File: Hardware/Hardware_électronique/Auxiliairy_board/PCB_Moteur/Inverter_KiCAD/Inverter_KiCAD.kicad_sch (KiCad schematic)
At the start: 67 parts, among them J1 Conn_02x02_Top_Bottom, J2 173010542, J3 Conn_02x05_Odd_Even, J4 Conn_01x02, J5 Conn_01x02, Q5 SQ2310ES, U1 MIC4606, U2 GO 10-SME/SP3, U3 GO 10-SME/SP3, U4 AZ1117-3.3, U5 MAX3097ECSE+, U7 CSD86350Q5D, U8 CSD86350Q5D

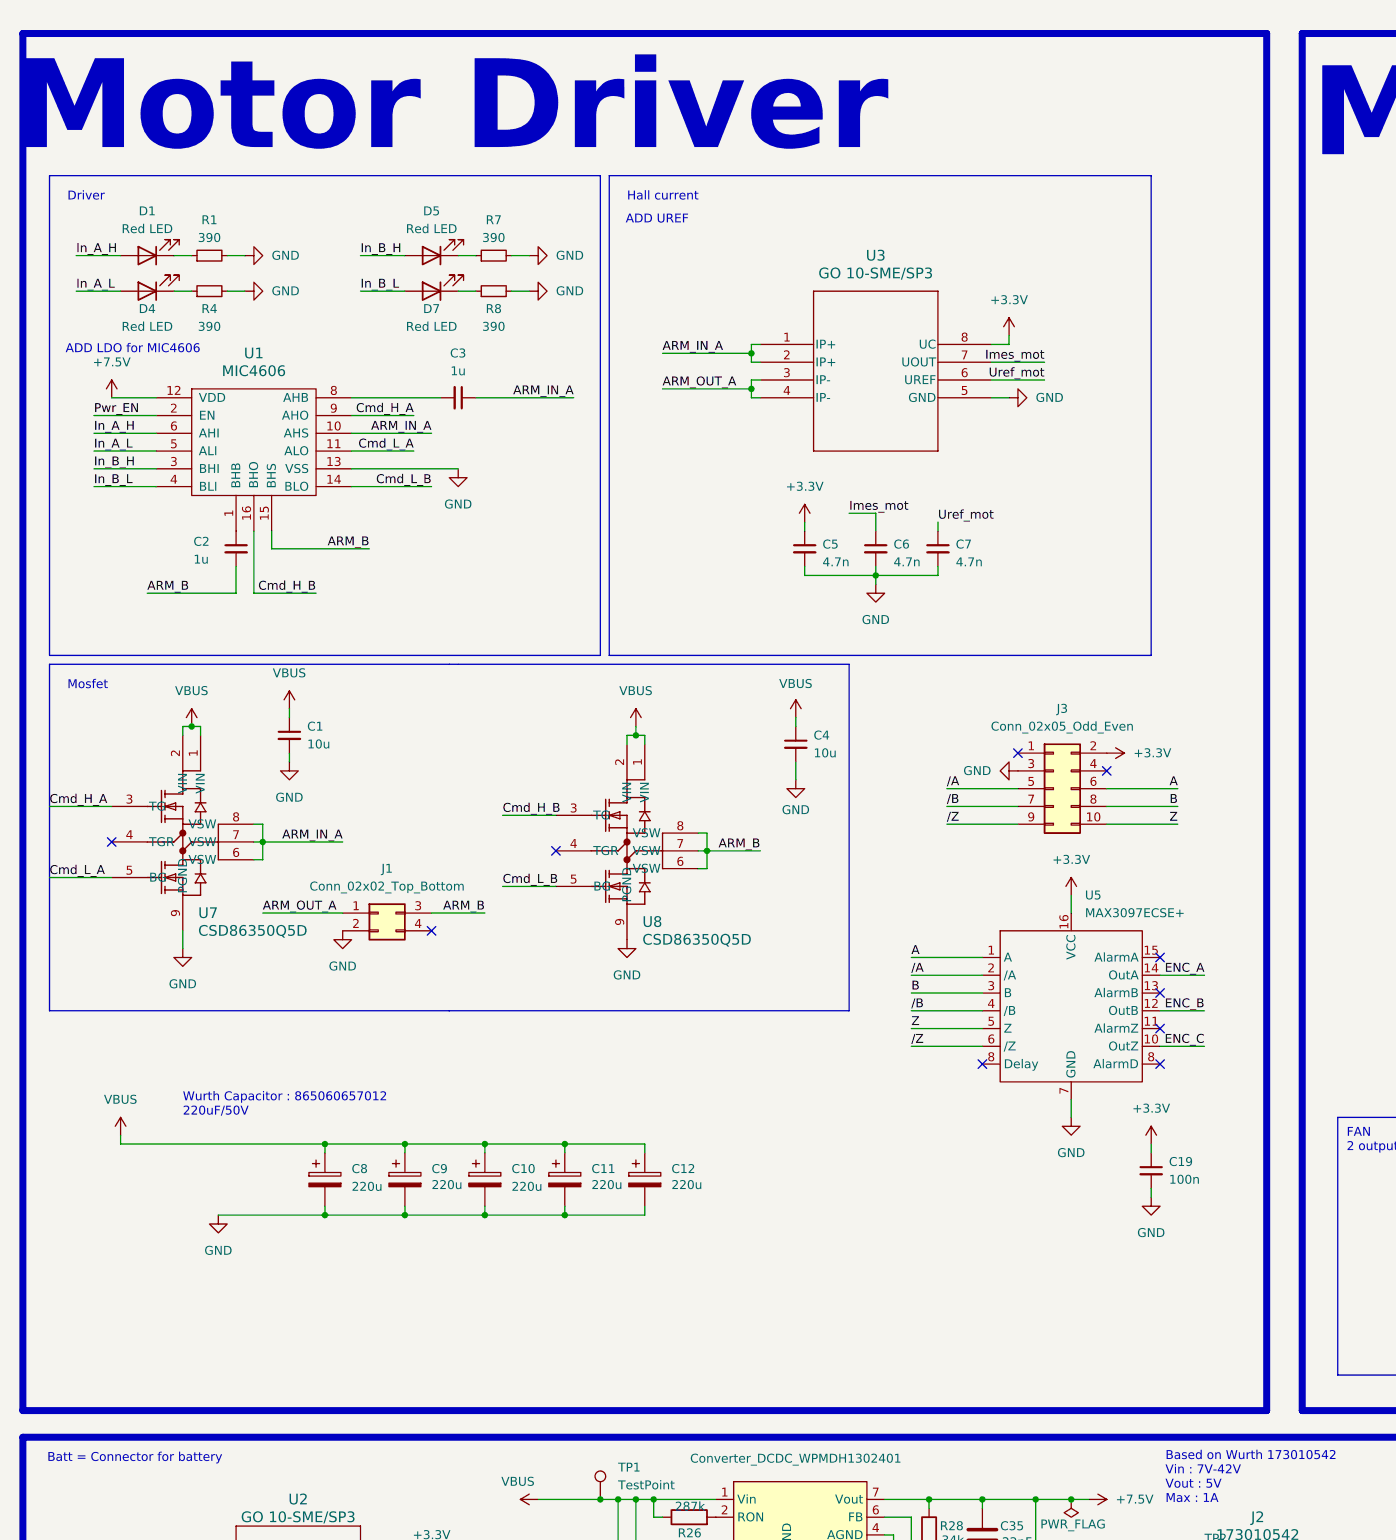
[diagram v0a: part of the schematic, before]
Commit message: ey
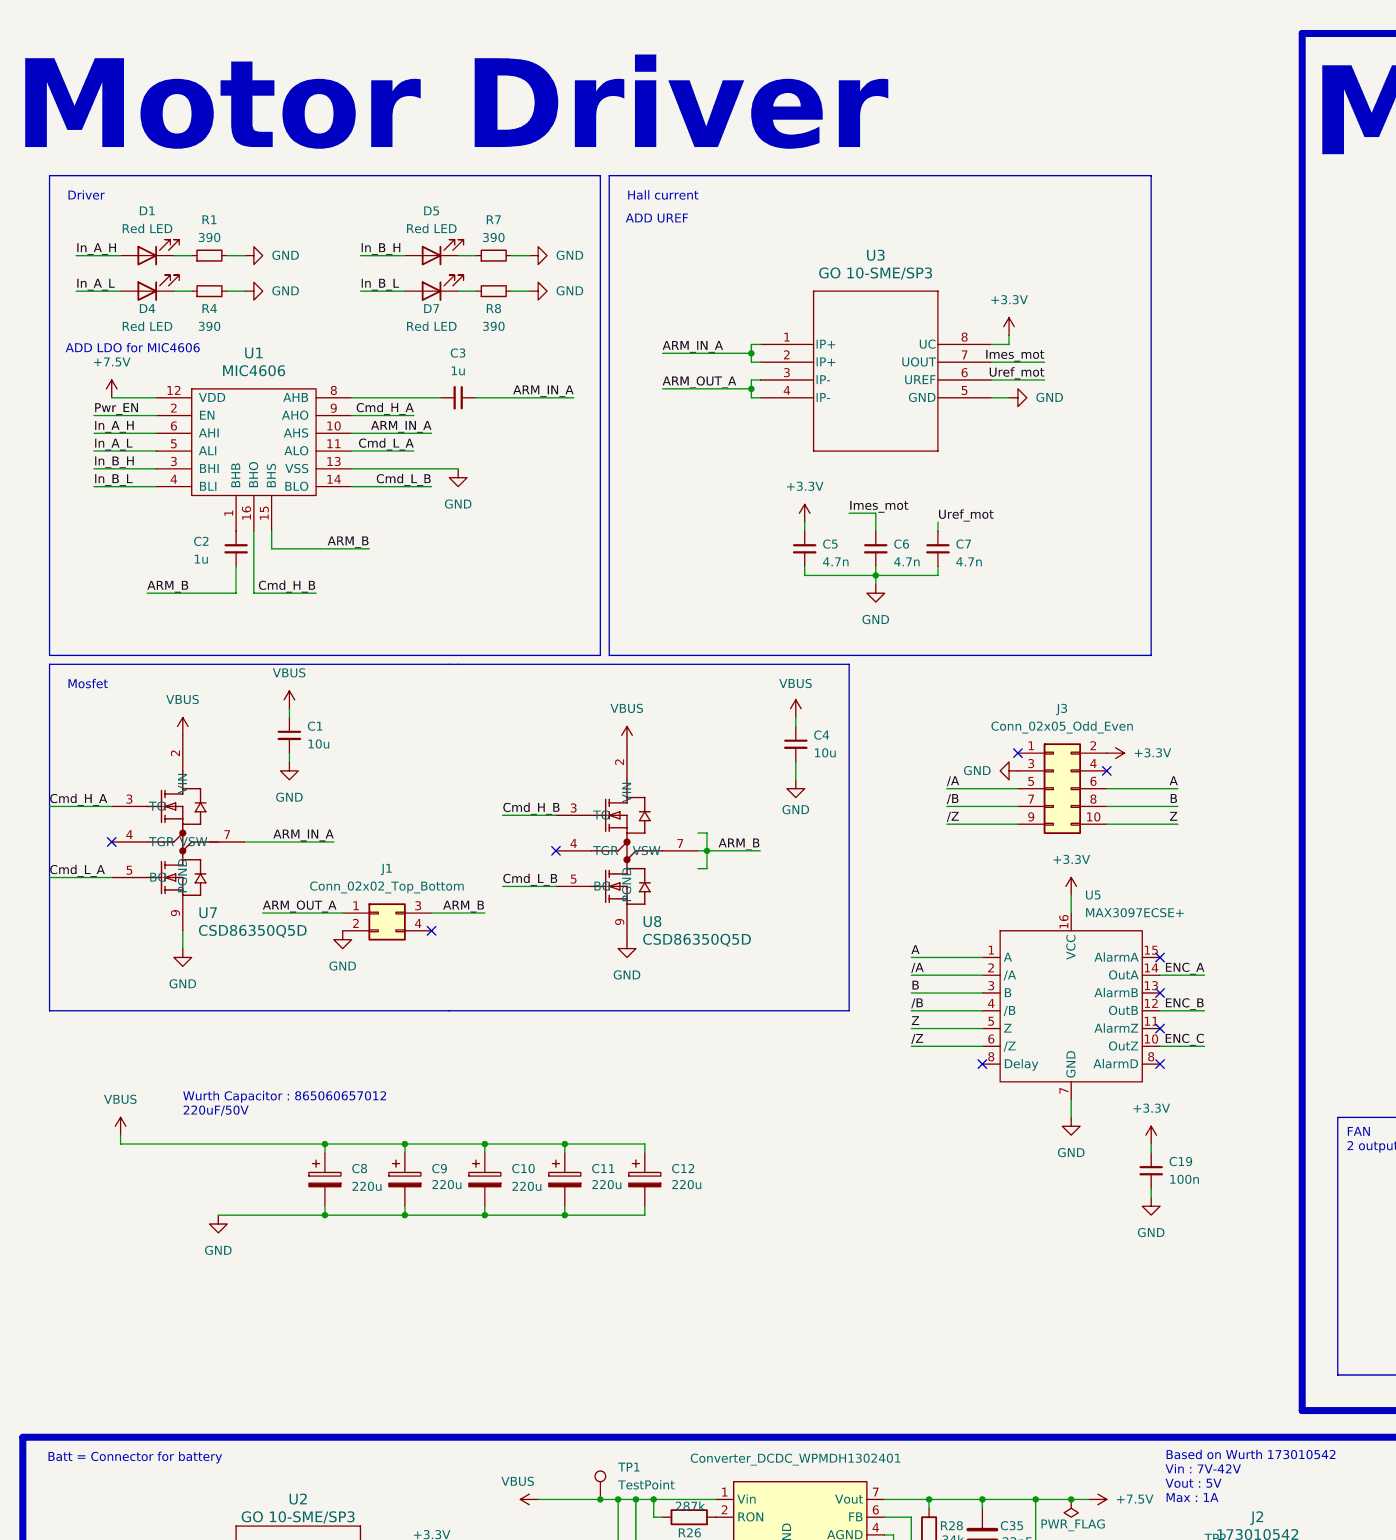
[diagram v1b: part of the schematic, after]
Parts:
- BT1: footprint Connector_AMASS:AMASS_XT60-F_1x02_P7.20mm_Vertical -> Connector_AMASS:AMASS_XT60-M_1x02_P7.20mm_Vertical
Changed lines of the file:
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@@
 	)
 	(junction
-		(at 102.87 114.3)
-		(diameter 0)
-		(color 0 0 0 0)
-	)
-	(junction
 		(at 92.71 172.72)
 		(diameter 0)
@@
 	)
 	(junction
-		(at 49.53 129.54)
-		(diameter 0)
-		(color 0 0 0 0)
-	)
-	(junction
 		(at 58.42 172.72)
 		(diameter 0)
@@
 	)
 	(junction
-		(at 39.37 113.03)
-		(diameter 0)
-		(color 0 0 0 0)
-	)
-	(junction
 		(at 332.74 241.3)
 		(diameter 0)
@@
 	(wire
 		(pts
-			(xy 40.64 113.03) (xy 40.64 114.3)
-		)
-		(stroke
-			(width 0)
-			(type default)
-		)
-	)
-	(wire
-		(pts
-			(xy 48.26 129.54) (xy 49.53 129.54)
+			(xy 46.99 129.54) (xy 59.69 129.54)
 		)
 		(stroke
@@
 	(wire
 		(pts
-			(xy 38.1 114.3) (xy 38.1 113.03)
-		)
-		(stroke
-			(width 0)
-			(type default)
-		)
-	)
-	(wire
-		(pts
 			(xy 252.73 181.61) (xy 254 181.61)
 		)
@@
 	(wire
 		(pts
-			(xy 49.53 129.54) (xy 60.96 129.54)
-		)
-		(stroke
-			(width 0)
-			(type default)
-		)
-	)
-	(wire
-		(pts
 			(xy 320.04 222.25) (xy 320.04 226.06)
 		)
@@
 	(wire
 		(pts
-			(xy 104.14 114.3) (xy 104.14 115.57)
-		)
-		(stroke
-			(width 0)
-			(type default)
-		)
-	)
-	(wire
-		(pts
 			(xy 50.8 87.63) (xy 64.77 87.63)
 		)
@@
 	(wire
 		(pts
-			(xy 49.53 132.08) (xy 49.53 129.54)
-		)
-		(stroke
-			(width 0)
-			(type default)
-		)
-	)
-	(wire
-		(pts
-			(xy 49.53 127) (xy 49.53 129.54)
-		)
-		(stroke
-			(width 0)
-			(type default)
-		)
-	)
-	(wire
-		(pts
 			(xy 58.42 182.88) (xy 69.85 182.88)
 		)
@@
 	(wire
 		(pts
-			(xy 102.87 113.03) (xy 102.87 114.3)
-		)
-		(stroke
-			(width 0)
-			(type default)
-		)
-	)
-	(wire
-		(pts
 			(xy 46.99 260.35) (xy 46.99 261.62)
 		)
@@
 	(wire
 		(pts
-			(xy 39.37 113.03) (xy 40.64 113.03)
-		)
-		(stroke
-			(width 0)
-			(type default)
-		)
-	)
-	(wire
-		(pts
 			(xy 81.28 182.88) (xy 92.71 182.88)
 		)
@@
 	(wire
 		(pts
-			(xy 101.6 114.3) (xy 102.87 114.3)
-		)
-		(stroke
-			(width 0)
-			(type default)
-		)
-	)
-	(wire
-		(pts
 			(xy 215.9 187.96) (xy 237.49 187.96)
 		)
@@
 	(wire
 		(pts
-			(xy 102.87 114.3) (xy 104.14 114.3)
-		)
-		(stroke
-			(width 0)
-			(type default)
-		)
-	)
-	(wire
-		(pts
 			(xy 53.34 110.49) (xy 53.34 111.76)
 		)
@@
 	(wire
 		(pts
-			(xy 101.6 115.57) (xy 101.6 114.3)
-		)
-		(stroke
-			(width 0)
-			(type default)
-		)
-	)
-	(wire
-		(pts
 			(xy 165.1 257.81) (xy 168.91 257.81)
 		)
@@
 	(wire
 		(pts
-			(xy 48.26 132.08) (xy 49.53 132.08)
-		)
-		(stroke
-			(width 0)
-			(type default)
-		)
-	)
-	(wire
-		(pts
 			(xy 168.91 269.24) (xy 182.88 269.24)
 		)
@@
 	(wire
 		(pts
-			(xy 38.1 113.03) (xy 39.37 113.03)
-		)
-		(stroke
-			(width 0)
-			(type default)
-		)
-	)
-	(wire
-		(pts
 			(xy 106.68 64.77) (xy 119.38 64.77)
 		)
@@
 	(wire
 		(pts
-			(xy 48.26 127) (xy 49.53 127)
-		)
-		(stroke
-			(width 0)
-			(type default)
-		)
-	)
-	(wire
-		(pts
 			(xy 92.71 181.61) (xy 92.71 182.88)
 		)
@@
 	)
 	(rectangle
-		(start 15.24 13.97)
-		(end 193.04 210.82)
-		(stroke
-			(width 1)
-			(type default)
-		)
-		(fill
-			(type color)
-			(color 255 246 235 1)
-		)
-	)
-	(rectangle
 		(start 303.53 168.91)
 		(end 400.05 205.74)
@@
 	)
 	(label "ARM_IN_A"
-		(at 60.96 129.54 180)
+		(at 59.69 129.54 180)
 		(fields_autoplaced yes)
 		(effects
@@
 	)
 	(symbol
+		(lib_name "CSD86350Q5D_1")
 		(lib_id "CSD87351Q5D:CSD86350Q5D")
 		(at 38.1 129.54 0)
@@
 		)
 		(property "Footprint" "CSD87351Q5D:DQY0008A"
-			(at 38.1 129.54 0)
+			(at 52.832 116.586 0)
 			(effects
 				(font
@@
 		)
 		(property "Datasheet" "CSD86350Q5D"
-			(at 38.1 129.54 0)
+			(at 47.752 118.618 0)
 			(effects
 				(font
@@
 		)
 		(property "Footprint" "CSD87351Q5D:DQY0008A"
-			(at 101.6 130.81 0)
+			(at 110.998 118.872 0)
 			(effects
 				(font
@@
 		)
 		(property "Datasheet" "CSD86350Q5D"
-			(at 101.6 130.81 0)
+			(at 110.998 120.904 0)
 			(effects
 				(font
@@
 			)
 		)
-		(property "Footprint" "Connector_AMASS:AMASS_XT60-F_1x02_P7.20mm_Vertical"
+		(property "Footprint" "Connector_AMASS:AMASS_XT60-M_1x02_P7.20mm_Vertical"
 			(at 22.86 242.316 90)
 			(effects
@@
 	(symbol
 		(lib_id "power:VBUS")
-		(at 39.37 113.03 0)
+		(at 38.1 114.3 0)
 		(unit 1)
 		(exclude_from_sim no)
@@
 		(fields_autoplaced yes)
 		(property "Reference" "#PWR048"
-			(at 39.37 116.84 0)
+			(at 38.1 118.11 0)
 			(effects
 				(font
@@
 		)
 		(property "Value" "VBUS"
-			(at 39.37 107.95 0)
+			(at 38.1 109.22 0)
 			(effects
 				(font
@@
 		)
 		(property "Footprint" ""
-			(at 39.37 113.03 0)
+			(at 38.1 114.3 0)
 			(effects
 				(font
@@
 		)
 		(property "Datasheet" ""
-			(at 39.37 113.03 0)
+			(at 38.1 114.3 0)
 			(effects
 				(font
@@
 		)
 		(property "Description" "Power symbol creates a global label with name \"VBUS\""
-			(at 39.37 113.03 0)
+			(at 38.1 114.3 0)
 			(effects
 				(font
@@
 	(symbol
 		(lib_id "power:VBUS")
-		(at 102.87 113.03 0)
+		(at 101.6 115.57 0)
 		(unit 1)
 		(exclude_from_sim no)
@@
 		(fields_autoplaced yes)
 		(property "Reference" "#PWR047"
-			(at 102.87 116.84 0)
+			(at 101.6 119.38 0)
 			(effects
 				(font
@@
 		)
 		(property "Value" "VBUS"
-			(at 102.87 107.95 0)
+			(at 101.6 110.49 0)
 			(effects
 				(font
@@
 		)
 		(property "Footprint" ""
-			(at 102.87 113.03 0)
+			(at 101.6 115.57 0)
 			(effects
 				(font
@@
 		)
 		(property "Datasheet" ""
-			(at 102.87 113.03 0)
+			(at 101.6 115.57 0)
 			(effects
 				(font
@@
 		)
 		(property "Description" "Power symbol creates a global label with name \"VBUS\""
-			(at 102.87 113.03 0)
+			(at 101.6 115.57 0)
 			(effects
 				(font
